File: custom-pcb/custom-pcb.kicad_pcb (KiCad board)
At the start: 2 copper layers, 72.4 x 72.4 mm, 68 parts, among them J1 CONN_CTL, J2 CONN_UART, J3 CONN_DBRD_IN, J4 CONN_DBRD_OUT, SW1 RESET, SW10 RESET_D, SW11 BOOT_D, SW2 BOOT, SW3 SPR_POWER, SW4 SPR_FAN, SW5 SPR_NIGHT, SW6 SPR_TIMER, SW7 SPR_FILTER, SW8 SPR_LIGHT, SW9 SPR_LOCK, U1 AMS1117-3.3, U2 74HCT595PW,118, U3 74HCT595PW,118, U4 ESP32-WROOM-32

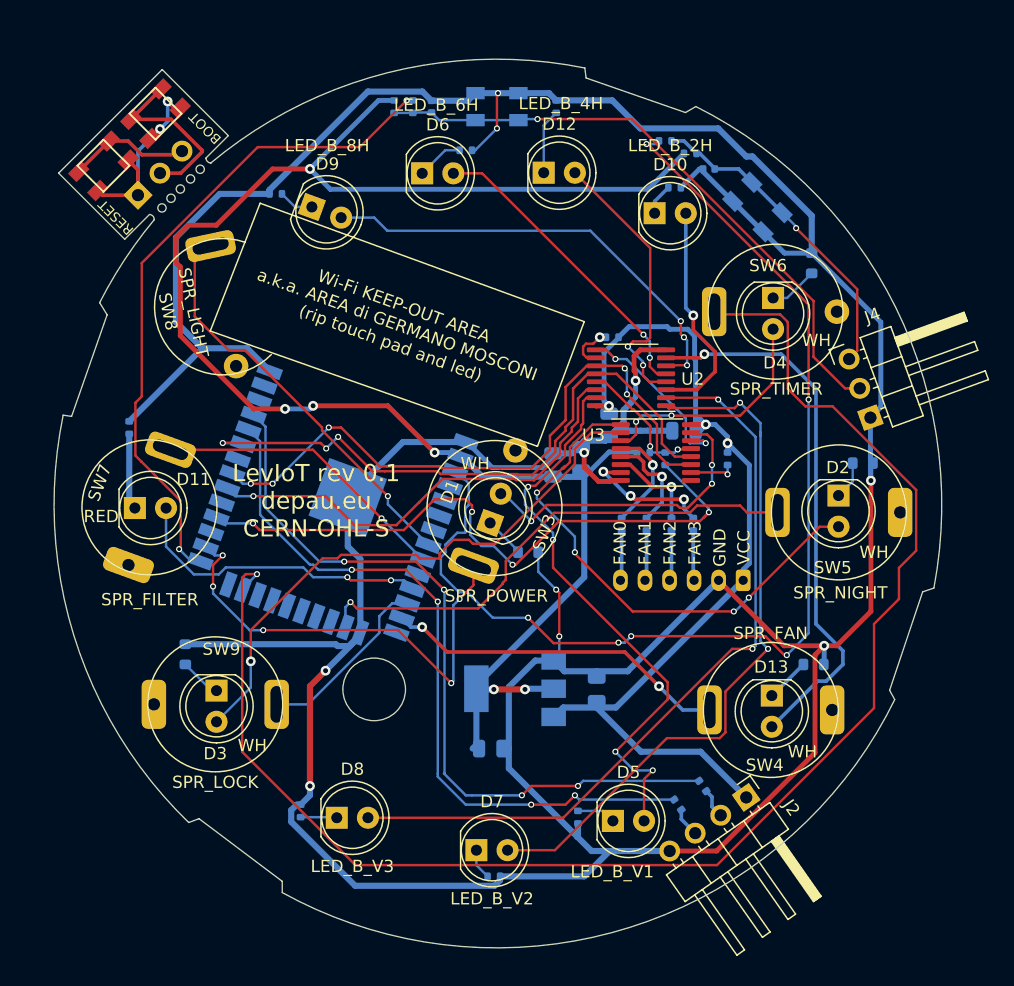
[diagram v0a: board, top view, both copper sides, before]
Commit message: Latest changes
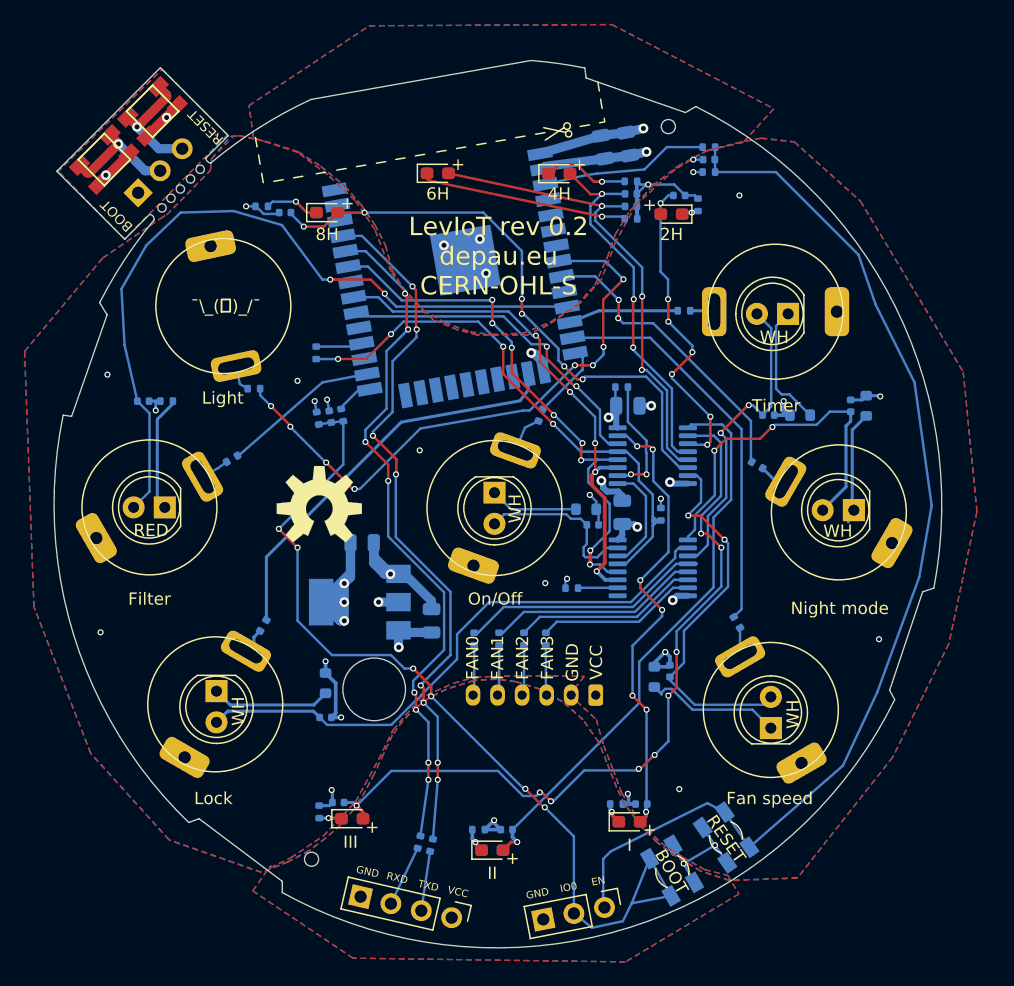
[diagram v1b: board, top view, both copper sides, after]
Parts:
- added ?: , custom-pcb:OSHW-LOGO-L, F.Cu at (99.6, 81.5)
- added C10: 0u1, Capacitor_SMD:C_0402_1005Metric, B.Cu at (142.9, 73.2)
- added C11: 0u1, Capacitor_SMD:C_0402_1005Metric, B.Cu at (100.1, 98.6)
- added C12: 0u1, Capacitor_SMD:C_0402_1005Metric, B.Cu at (136.2, 73.9)
- added C13: 0u1, Capacitor_SMD:C_0402_1005Metric, B.Cu at (125.8, 105.6)
- added C14: 0u1, Capacitor_SMD:C_0402_1005Metric, B.Cu at (125.0, 56.9)
- added C15: 0u1, Capacitor_SMD:C_0402_1005Metric, B.Cu at (114.8, 107.7)
- added C16: 0u1, Capacitor_SMD:C_0402_1005Metric, B.Cu at (96.8, 57.4)
- added C17: 0u1, Capacitor_SMD:C_0402_1005Metric, B.Cu at (101.1, 105.5)
- added C18: 0u1, Capacitor_SMD:C_0402_1005Metric, B.Cu at (128.1, 94.8)
- added C19: 0u1, Capacitor_SMD:C_0402_1005Metric, B.Cu at (128.9, 56.0)
- added C20: 0u1, Capacitor_SMD:C_0402_1005Metric, B.Cu at (125.0, 55.9)
- added C21: 0u1, Capacitor_SMD:C_0402_1005Metric, B.Cu at (85.2, 72.8)
- added C9: 0u1, Capacitor_SMD:C_0402_1005Metric, B.Cu at (121.8, 82.9)
- added R28: 510R, Resistor_SMD:R_0402_1005Metric, B.Cu at (117.6, 73.9)
- added R29: 510R, Resistor_SMD:R_0402_1005Metric, B.Cu at (133.6, 90.8)
- added R30: 510R, Resistor_SMD:R_0402_1005Metric, B.Cu at (135.3, 78.0)
- added R31: 510R, Resistor_SMD:R_0402_1005Metric, B.Cu at (129.3, 65.4)
- added R32: 510R, Resistor_SMD:R_0402_1005Metric, B.Cu at (92.5, 77.5)
- added R33: 510R, Resistor_SMD:R_0402_1005Metric, B.Cu at (94.2, 71.8)
- added R34: 510R, Resistor_SMD:R_0402_1005Metric, B.Cu at (95.0, 91.1)
- added REF**: ToolingHole_1.152mm_(for_JLCPCB_SMT), custom-pcb:ToolingHole_1.152mm_(for_JLCPCB_SMT), F.Cu at (128.0, 50.4)
- added REF**: ToolingHole_1.152mm_(for_JLCPCB_SMT), custom-pcb:ToolingHole_1.152mm_(for_JLCPCB_SMT), F.Cu at (98.9, 110.1)
- C5: value 0u1 -> 10u
- D1: value LED_W_POWER -> On/Off; footprint LED_THT:LED_D5.0mm -> custom-pcb:LED_D5.0mm-centered
- D10: value LED_B_2H -> 2H; footprint LED_THT:LED_D5.0mm -> LED_SMD:LED_0603_1608Metric_Pad1.05x0.95mm_HandSolder
- D11, D13, D2, D3, D4: footprint LED_THT:LED_D5.0mm -> custom-pcb:LED_D5.0mm-centered
- D12: value LED_B_4H -> 4H; footprint LED_THT:LED_D5.0mm -> LED_SMD:LED_0603_1608Metric_Pad1.05x0.95mm_HandSolder
- D5: value LED_B_V1 -> I; footprint LED_THT:LED_D5.0mm -> LED_SMD:LED_0603_1608Metric_Pad1.05x0.95mm_HandSolder
- D6: value LED_B_6H -> 6H; footprint LED_THT:LED_D5.0mm -> LED_SMD:LED_0603_1608Metric_Pad1.05x0.95mm_HandSolder
- D7: value LED_B_V2 -> II; footprint LED_THT:LED_D5.0mm -> LED_SMD:LED_0603_1608Metric_Pad1.05x0.95mm_HandSolder
- D8: value LED_B_V3 -> III; footprint LED_THT:LED_D5.0mm -> LED_SMD:LED_0603_1608Metric_Pad1.05x0.95mm_HandSolder
- D9: value LED_B_8H -> 8H; footprint LED_THT:LED_D5.0mm -> LED_SMD:LED_0603_1608Metric_Pad1.05x0.95mm_HandSolder
- J2: footprint Connector_PinHeader_2.54mm:PinHeader_1x04_P2.54mm_Horizontal -> Connector_PinHeader_2.54mm:PinHeader_1x04_P2.54mm_Vertical
- J4: footprint Connector_PinHeader_2.54mm:PinHeader_1x03_P2.54mm_Horizontal -> Connector_PinHeader_2.54mm:PinHeader_1x03_P2.54mm_Vertical
- SW4: value SPR_FAN -> Fan speed
- SW5: value SPR_NIGHT -> Night mode
- SW6: value SPR_TIMER -> Timer
- SW7: value SPR_FILTER -> Filter
- SW8: value SPR_LIGHT -> Light; footprint touchpad_spring:touchpad_sprint_nosilk -> touchpad_spring:touchpad_spring
- SW9: value SPR_LOCK -> Lock
- U2, U3: moved to B.Cu
- moved SW2 63.9 mm to (128.3, 111.0), turned to -60 degrees
- moved SW1 51.4 mm to (132.7, 108.3), turned to -55 degrees
- moved J4 48.9 mm to (122.8, 114.0), turned to -79 degrees
- moved R25 29.7 mm to (99.3, 68.8), turned to -90 degrees
- moved C6 26.6 mm to (100.5, 74.0), turned to 100 degrees
- moved C8 26.2 mm to (122.7, 52.1), turned to 100 degrees
- moved R15 26.1 mm to (99.4, 74.2), turned to -80 degrees
- moved J2 25.9 mm to (110.4, 114.9), turned to -103 degrees
- moved C7 25.9 mm to (124.7, 51.8), turned to 100 degrees
- moved R21 25.8 mm to (101.4, 73.9), turned to 100 degrees
- moved R23 22.6 mm to (108.7, 109.0), turned to 77 degrees
- moved R24 21.3 mm to (107.7, 108.7), turned to 77 degrees
- moved U4 21.2 mm to (110.6, 62.2), turned to -170 degrees
- moved C4 19.8 mm to (103.1, 84.3)
- moved R2 16.5 mm to (120.1, 88.0), turned to 180 degrees
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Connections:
- SW3 pad 1: TOUCH_POWER -> Net-(R28-Pad1)
- SW4 pad 1: TOUCH_FAN -> Net-(R29-Pad1)
- SW5 pad 1: TOUCH_NIGHT -> Net-(R30-Pad1)
- SW6 pad 1: TOUCH_TIMER -> Net-(R31-Pad1)
- SW7 pad 1: TOUCH_FILTER -> Net-(R32-Pad1)
- SW8 pad 1: TOUCH_LIGHT -> Net-(R33-Pad1)
- SW9 pad 1: TOUCH_LOCK -> Net-(R34-Pad1)
- U4 pad 12: TOUCH_LOCK -> TOUCH_TIMER
- U4 pad 14: (no net) -> TOUCH_POWER
- U4 pad 16: TOUCH_NIGHT -> TOUCH_LOCK
- U4 pad 23: TOUCH_TIMER -> (no net)
- U4 pad 26: TOUCH_POWER -> TOUCH_FILTER
- U4 pad 9: TOUCH_FILTER -> TOUCH_NIGHT
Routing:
- net GND: track 365.7 -> 226.0 mm, vias 10 -> 34
- net TOUCH_TIMER: track 122.8 -> 9.43 mm, vias 1 -> 0
- net Net-(R17-Pad1): track 90.7 -> 13.7 mm, vias 6 -> 0
- net EN: track 26.2 -> 89.3 mm, vias 1 -> 0
- net Net-(R21-Pad2): track 54.8 -> 3.07 mm, vias 2 -> 0
- net Net-(R25-Pad1): track 53.2 -> 3.82 mm, vias 4 -> 0
- net LED_RED_FILTER: track 25.1 -> 62.1 mm
- net SHIFT_OUTEN: track 11.9 -> 47.3 mm, vias 2 -> 4
- net TOUCH_POWER: track 37.9 -> 6.35 mm, vias 5 -> 0
- net IO0: track 50.0 -> 74.6 mm, vias 1 -> 6
- net TOUCH_LOCK: track 14.8 -> 33.0 mm
- net TOUCH_NIGHT: track 41.9 -> 24.6 mm, vias 1 -> 2
- net TOUCH_LIGHT: track 33.5 -> 48.5 mm, vias 1 -> 8
- net LED_BLUE_6H: track 25.3 -> 39.4 mm, vias 2 -> 3
- net LED_WHITE_FAN: track 44.8 -> 31.3 mm, vias 1 -> 2
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- added copper zone on B.Cu, net GND
- added copper zone on F.Cu, net GND
- added copper zone on In2.Cu, net GND
- added copper zone on B.Cu, net GND1
- added copper zone on F.Cu, net GND1
- added copper zone on In2.Cu, net GND1
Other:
- board size 72.4 x 72.4 mm -> 72.4 x 72.3 mm
- copper layers 2 -> 4
- net class Default removed
- board text added: "+"
- board text added: "DBOARD"
- board text added: "LevIoT rev 0.2 depau.eu CERN-OHL-S"
- board text added: "¯\_(ツ)_/¯"
- board text removed: "BUTTONS DBRD"
- board text removed: "LED 2H"
- board text removed: "LED 4H"
- board text removed: "LED 6H"
- board text removed: "LED 8H"
- board text removed: "LED V1"
- board text removed: "LED V2"
- board text removed: "LED V3"
- board text removed: "LevIoT rev 0.1 depau.eu CERN-OHL-S"
- board text removed: "Wi-Fi KEEP-OUT AREA a.k.a. AREA di GERMANO MOSCONI"
- board text removed: "Wi-Fi KEEP-OUT AREA a.k.a. AREA di GERMANO MOSCONI (rip touch pad and led)"
